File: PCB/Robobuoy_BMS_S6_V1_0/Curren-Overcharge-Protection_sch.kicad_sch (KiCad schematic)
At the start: 23 parts, among them Q201 AO3400A, Q203 AO3400A, Q204 HYG025N04NA1C2, Q205 HYG025N04NA1C2, Q206 HYG025N04NA1C2, Q207 HYG025N04NA1C2, Q208 AO3400A, Q209 AO3400A

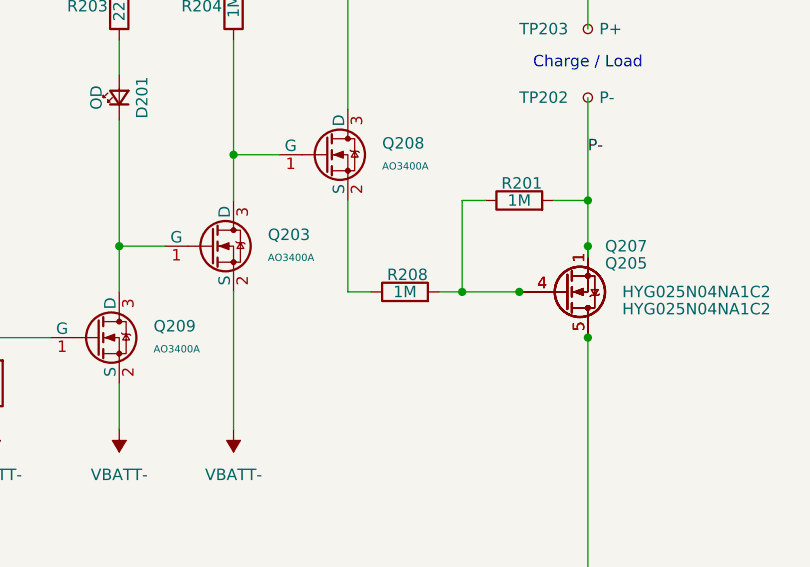
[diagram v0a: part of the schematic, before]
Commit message: PCB adjustmend Sub V3.0
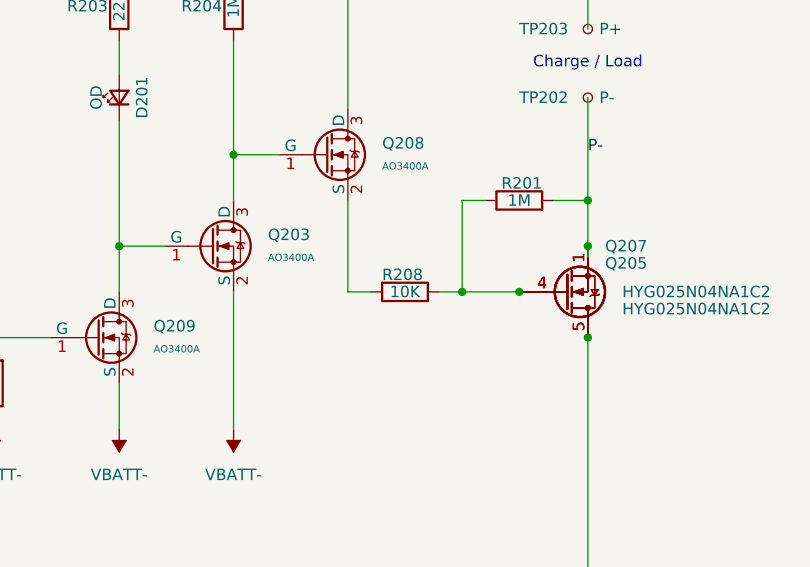
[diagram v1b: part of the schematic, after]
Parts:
- R208: value 1M -> 10K; LCSC C22935 -> (none)
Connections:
- net at Q205.4 (G), Q207.4 (G), R201.1: now also R208.1; no longer R208.2
- net at Q208.2 (S): now also R208.2; no longer R208.1
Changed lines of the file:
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@@
+	)
+	(symbol
+		(lib_id "Device:R")
+		(at 135.89 59.69 270)
+		(unit 1)
+		(exclude_from_sim no)
+		(in_bom yes)
+		(on_board yes)
+		(dnp no)
+		(property "Reference" "R208"
+			(at 133.35 57.785 90)
+			(effects
+				(font
+					(size 1.27 1.27)
+				)
+				(justify left)
+			)
+		)
+		(property "Value" "10K"
+			(at 135.89 59.69 90)
+			(effects
+				(font
+					(size 1.27 1.27)
+				)
+			)
+		)
+		(property "Footprint" "A_Device:R_0603"
+			(at 135.89 57.912 90)
+			(effects
+				(font
+					(size 1.27 1.27)
+				)
+				(hide yes)
+			)
+		)
+		(property "Datasheet" ""
+			(at 135.89 59.69 0)
+			(effects
+				(font
+					(size 1.27 1.27)
+				)
+				(hide yes)
+			)
+		)
+		(property "Description" ""
+			(at 135.89 59.69 0)
+			(effects
+				(font
+					(size 1.27 1.27)
+				)
+				(hide yes)
+			)
+		)
+		(property "LCSC" ""
+			(at 135.89 59.69 0)
+			(effects
+				(font
+					(size 1.27 1.27)
+				)
+				(hide yes)
+			)
+		)
+		(property "Collector Current (Ic)" ""
+			(at 135.89 59.69 0)
+			(effects
+				(font
+					(size 1.27 1.27)
+				)
+				(hide yes)
+			)
+		)
+		(property "Collector Cut-Off Current (Icbo)" ""
+			(at 135.89 59.69 0)
+			(effects
+				(font
+					(size 1.27 1.27)
+				)
+				(hide yes)
+			)
+		)
+		(property "Collector-Emitter Breakdown Voltage (Vceo)" ""
+			(at 135.89 59.69 0)
+			(effects
+				(font
+					(size 1.27 1.27)
+				)
+				(hide yes)
+			)
+		)
+		(property "Collector-Emitter Saturation Voltage (VCE(sat)@Ic,Ib)" ""
+			(at 135.89 59.69 0)
+			(effects
+				(font
+					(size 1.27 1.27)
+				)
+				(hide yes)
+			)
+		)
+		(property "DC Current Gain (hFE@Ic,Vce)" ""
+			(at 135.89 59.69 0)
+			(effects
+				(font
+					(size 1.27 1.27)
+				)
+				(hide yes)
+			)
+		)
+		(property "Sim.Device" ""
+			(at 135.89 59.69 0)
+			(effects
+				(font
+					(size 1.27 1.27)
+				)
+				(hide yes)
+			)
+		)
+		(property "Sim.Type" ""
+			(at 135.89 59.69 0)
+			(effects
+				(font
+					(size 1.27 1.27)
+				)
+				(hide yes)
+			)
+		)
+		(property "Transistor Type" ""
+			(at 135.89 59.69 0)
+			(effects
+				(font
+					(size 1.27 1.27)
+				)
+				(hide yes)
+			)
+		)
+		(property "Transition Frequency (fT)" ""
+			(at 135.89 59.69 0)
+			(effects
+				(font
+					(size 1.27 1.27)
+				)
+				(hide yes)
+			)
+		)
+		(pin "1"
+		)
+		(pin "2"
+		)
+		(instances
+			(project "Robobuoy_BMS_S6_V1_0"
+				(path "/1f52533e-1c9e-4a55-ac43-3d9bafbde785/56ee7f72-20af-47b1-badb-ded1b77856b8"
+					(reference "R208")
+					(unit 1)
+				)
+			)
+		)
 	)
 	(symbol
@@
 					(unit 1)
 				)
-			)
-		)
-	)
-	(symbol
-		(lib_id "Device:R")
-		(at 135.89 59.69 90)
-		(unit 1)
-		(exclude_from_sim no)
-		(in_bom yes)
-		(on_board yes)
-		(dnp no)
-		(property "Reference" "R208"
-			(at 138.43 57.785 90)
-			(effects
-				(font
-					(size 1.27 1.27)
-				)
-				(justify left)
-			)
-		)
-		(property "Value" "1M"
-			(at 135.89 59.69 90)
-			(effects
-				(font
-					(size 1.27 1.27)
-				)
-			)
-		)
-		(property "Footprint" "A_Device:R_0603"
-			(at 135.89 61.468 90)
-			(effects
-				(font
-					(size 1.27 1.27)
-				)
-				(hide yes)
-			)
-		)
-		(property "Datasheet" ""
-			(at 135.89 59.69 0)
-			(effects
-				(font
-					(size 1.27 1.27)
-				)
-				(hide yes)
-			)
-		)
-		(property "Description" ""
-			(at 135.89 59.69 0)
-			(effects
-				(font
-					(size 1.27 1.27)
-				)
-				(hide yes)
-			)
-		)
-		(property "LCSC" "C22935"
-			(at 135.89 59.69 0)
-			(effects
-				(font
-					(size 1.27 1.27)
-				)
-				(hide yes)
-			)
-		)
-		(property "MF" ""
-			(at 135.89 59.69 0)
-			(effects
-				(font
-					(size 1.27 1.27)
-				)
-				(hide yes)
-			)
-		)
-		(property "MFN" ""
-			(at 135.89 59.69 0)
-			(effects
-				(font
-					(size 1.27 1.27)
-				)
-				(hide yes)
-			)
-		)
-		(property "info" ""
-			(at 135.89 59.69 0)
-			(effects
-				(font
-					(size 1.27 1.27)
-				)
-				(hide yes)
-			)
-		)
-		(property "Collector Current (Ic)" ""
-			(at 135.89 59.69 0)
-			(effects
-				(font
-					(size 1.27 1.27)
-				)
-				(hide yes)
-			)
-		)
-		(property "Collector Cut-Off Current (Icbo)" ""
-			(at 135.89 59.69 0)
-			(effects
-				(font
-					(size 1.27 1.27)
-				)
-				(hide yes)
-			)
-		)
-		(property "Collector-Emitter Breakdown Voltage (Vceo)" ""
-			(at 135.89 59.69 0)
-			(effects
-				(font
-					(size 1.27 1.27)
-				)
-				(hide yes)
-			)
-		)
-		(property "Collector-Emitter Saturation Voltage (VCE(sat)@Ic,Ib)" ""
-			(at 135.89 59.69 0)
-			(effects
-				(font
-					(size 1.27 1.27)
-				)
-				(hide yes)
-			)
-		)
-		(property "DC Current Gain (hFE@Ic,Vce)" ""
-			(at 135.89 59.69 0)
-			(effects
-				(font
-					(size 1.27 1.27)
-				)
-				(hide yes)
-			)
-		)
-		(property "Sim.Device" ""
-			(at 135.89 59.69 0)
-			(effects
-				(font
-					(size 1.27 1.27)
-				)
-				(hide yes)
-			)
-		)
-		(property "Sim.Type" ""
-			(at 135.89 59.69 0)
-			(effects
-				(font
-					(size 1.27 1.27)
-				)
-				(hide yes)
-			)
-		)
-		(property "Transistor Type" ""
-			(at 135.89 59.69 0)
-			(effects
-				(font
-					(size 1.27 1.27)
-				)
-				(hide yes)
-			)
-		)
-		(property "Transition Frequency (fT)" ""
-			(at 135.89 59.69 0)
-			(effects
-				(font
-					(size 1.27 1.27)
-				)
-				(hide yes)
-			)
-		)
-		(pin "1"
-		)
-		(pin "2"
-		)
-		(instances
-			(project "Robobuoy_BMS_S6_V1_0"
-				(path "/1f52533e-1c9e-4a55-ac43-3d9bafbde785/56ee7f72-20af-47b1-badb-ded1b77856b8"
-					(reference "R208")
-					(unit 1)
-				)
